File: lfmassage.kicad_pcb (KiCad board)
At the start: 2 copper layers, 63 x 55 mm, 47 parts, among them J1 Batt, J2 OUT, J3 ESP_DEVKITC, Q1 BFS20W, Q2 BC856B,215, Q3 BC856B,215, Q4 BC856B,215, Q5 BC856B,215, Q6 BC846,215, Q7 BC846,215, Q8 BC846,215, SW1 NW3-A03-05, SW2 SW_Push, SW3 SW_Push, SW4 SW_Push, U1 USB_CType_6Pin, U2 MCP73831

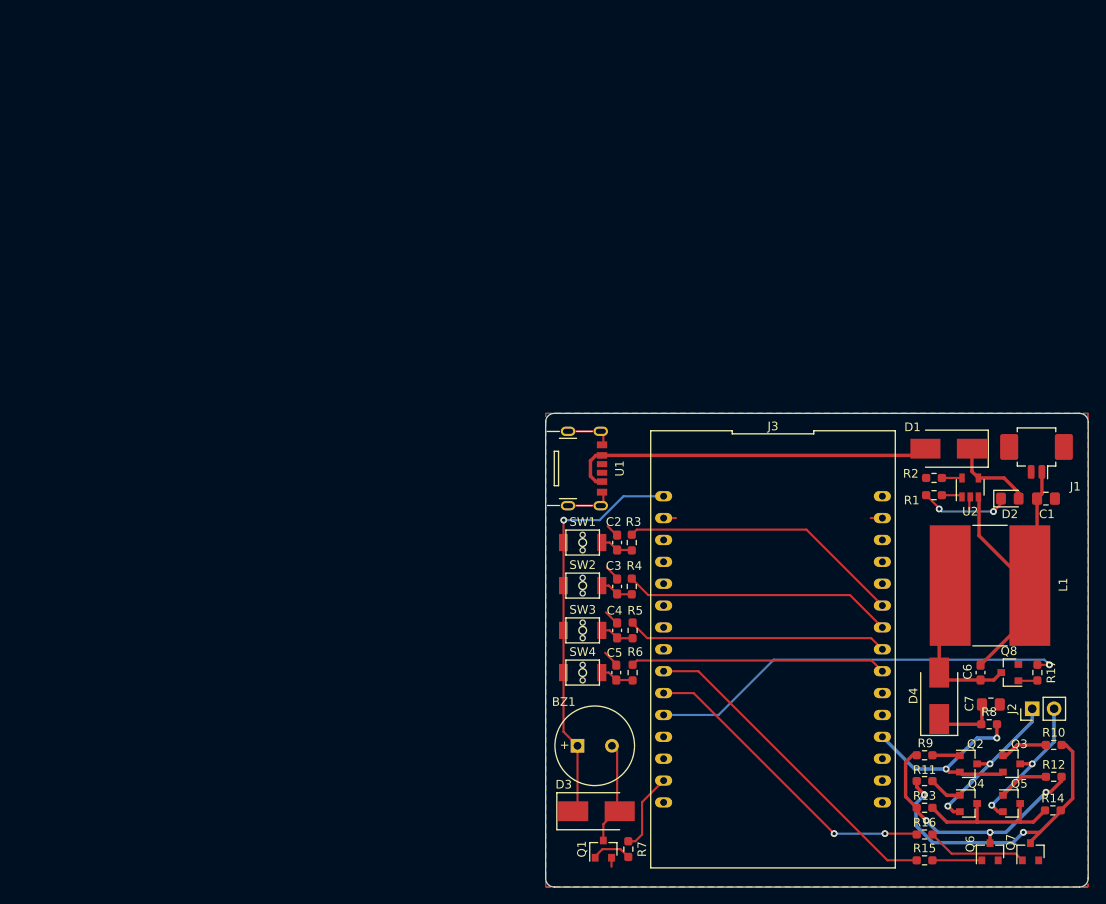
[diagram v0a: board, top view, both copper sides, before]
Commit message: 2021-09-26
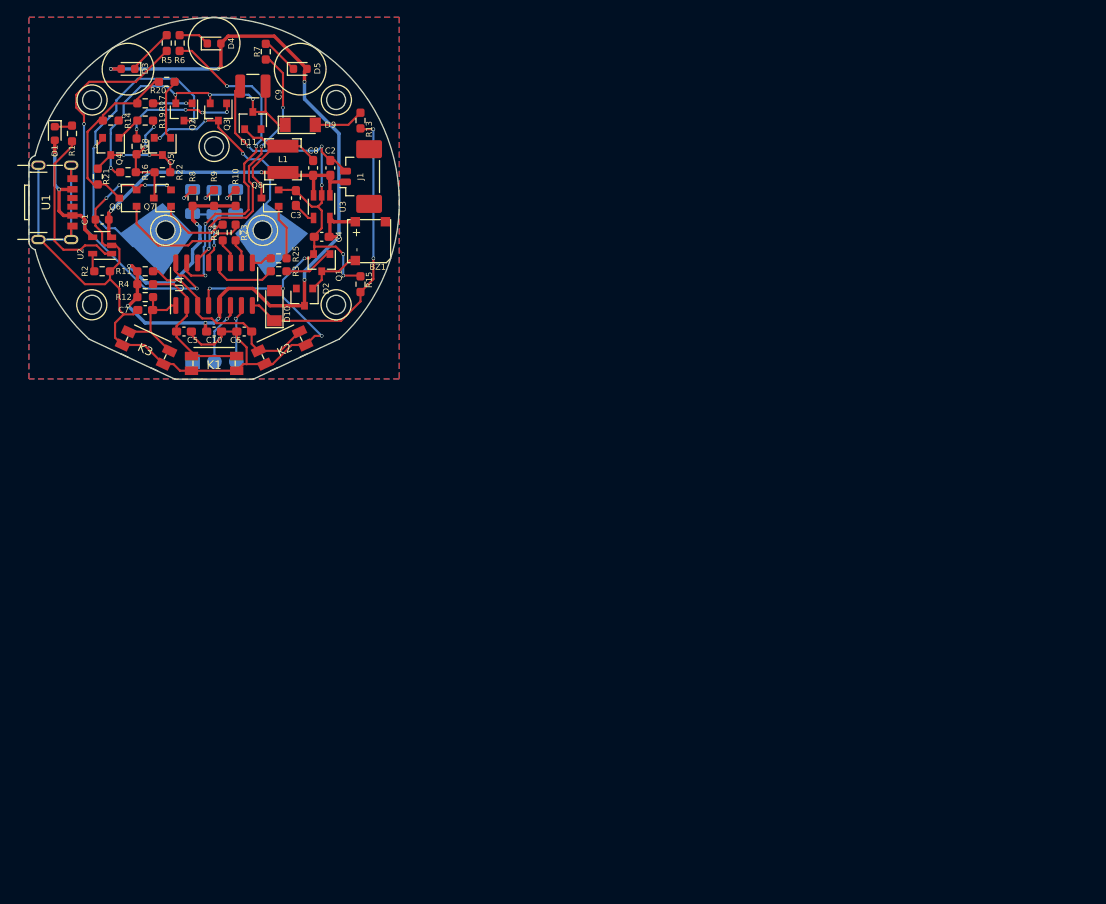
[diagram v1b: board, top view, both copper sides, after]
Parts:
- removed SW1: NW3-A03-05, ali_Switch:NW3-A03-05
- removed SW2, SW3, SW4: SW_Push, ali_Switch:NW3-A03-05
- added C10: 10uF/1608, Capacitor_SMD:C_0603_1608Metric_Pad1.08x0.95mm_HandSolder, F.Cu at (21.5, 36.5)
- added C8: 10nF, Capacitor_SMD:C_0603_1608Metric_Pad1.08x0.95mm_HandSolder, F.Cu at (33.0, 17.5)
- added C9: 10uF/3225, Capacitor_SMD:C_1210_3225Metric, F.Cu at (26.0, 8.00)
- added D10: Zenor/3.3V, Diode_SMD:D_MiniMELF, F.Cu at (28.5, 33.5)
- added D11: BAT54, Diode_SMD:D_SOT-23_ANK, F.Cu at (26.0, 12.0)
- added D5: LED/1608, LED_SMD:LED_0603_1608Metric, F.Cu at (31.5, 6.00)
- added D6: RED, LED_SMD:LED_1206_3216Metric, B.Cu at (19.0, 21.4)
- added D7: IR, LED_SMD:LED_1206_3216Metric, B.Cu at (21.5, 21.5)
- added D8: RED, LED_SMD:LED_1206_3216Metric, B.Cu at (24.0, 21.4)
- added D9: Zenor/47V, Diode_SMD:D_MiniMELF, F.Cu at (31.5, 12.5)
- added K1: MODE, Button_Switch_SMD:Panasonic_EVQPUJ_EVQPUA, F.Cu at (21.5, 40.2)
- added K2: +, Button_Switch_SMD:Panasonic_EVQPUJ_EVQPUA, F.Cu at (29.4, 38.4)
- added K3: -, Button_Switch_SMD:Panasonic_EVQPUJ_EVQPUA, F.Cu at (13.6, 38.4)
- added R18: 33k, Resistor_SMD:R_0603_1608Metric_Pad0.98x0.95mm_HandSolder, F.Cu at (12.5, 15.0)
- added R19: 33k, Resistor_SMD:R_0603_1608Metric_Pad0.98x0.95mm_HandSolder, F.Cu at (13.5, 12.0)
- added R20: 33k, Resistor_SMD:R_0603_1608Metric_Pad0.98x0.95mm_HandSolder, F.Cu at (16.0, 7.50)
- added R21: 33k, Resistor_SMD:R_0603_1608Metric_Pad0.98x0.95mm_HandSolder, F.Cu at (8.00, 18.5)
- added R22: 0, Resistor_SMD:R_0603_1608Metric_Pad0.98x0.95mm_HandSolder, F.Cu at (15.5, 18.0)
- added R23: 100, Resistor_SMD:R_0603_1608Metric_Pad0.98x0.95mm_HandSolder, F.Cu at (24.0, 25.0)
- added R24: 100, Resistor_SMD:R_0603_1608Metric_Pad0.98x0.95mm_HandSolder, F.Cu at (22.5, 25.0)
- added R25: 1k, Resistor_SMD:R_0603_1608Metric_Pad0.98x0.95mm_HandSolder, F.Cu at (29.0, 28.0)
- added REF**: MountingHole_2.2mm_M2, MountingHole:MountingHole_2.2mm_M2, F.Cu at (7.33, 33.4)
- added REF**: MountingHole_2.2mm_M2, MountingHole:MountingHole_2.2mm_M2, F.Cu at (7.33, 9.61)
- added REF**: MountingHole_2.2mm_M2, MountingHole:MountingHole_2.2mm_M2, F.Cu at (35.7, 33.4)
- added REF**: MountingHole_2.2mm_M2, MountingHole:MountingHole_2.2mm_M2, F.Cu at (35.7, 9.61)
- added REF**: MountingHole_2.2mm_M2, MountingHole:MountingHole_2.2mm_M2, F.Cu at (21.5, 15.0)
- added REF**: MountingHole_2.2mm_M2, MountingHole:MountingHole_2.2mm_M2, F.Cu at (27.1, 24.8)
- added REF**: MountingHole_2.2mm_M2, MountingHole:MountingHole_2.2mm_M2, F.Cu at (15.9, 24.8)
- added U3: MIC5318-2.8YD5-TR, Package_TO_SOT_SMD:TSOT-23-5, F.Cu at (34.0, 22.0)
- added U4: EFM8BB10F8G-A-SOIC16, Package_SO:SOIC-16_3.9x9.9mm_P1.27mm, F.Cu at (21.5, 31.0)
- BZ1: value IMT09B2703P -> BST-5533S; footprint Buzzer_Beeper:MagneticBuzzer_PUI_AT-0927-TT-6-R -> buzzer:BST-5533S
- C1: value 10uF/2012 -> 10uF/1608; footprint Capacitor_SMD:C_0805_2012Metric_Pad1.18x1.45mm_HandSolder -> Capacitor_SMD:C_0603_1608Metric
- C3: value 100nF/1608 -> 10nF/1608
- C6: value 10nF -> 100nF/1608
- C7: value 10uF/2012 -> 100nF/1608; footprint Capacitor_SMD:C_0805_2012Metric_Pad1.18x1.45mm_HandSolder -> Capacitor_SMD:C_0603_1608Metric_Pad1.08x0.95mm_HandSolder
- D1, D3, D4: value SK24/SMB -> LED/1608; footprint Diode_SMD:D_SMB_Handsoldering -> LED_SMD:LED_0603_1608Metric
- D2: value LED/2012 -> BAT54; footprint LED_SMD:LED_0805_2012Metric_Pad1.15x1.40mm_HandSolder -> Diode_SMD:D_SOT-23_ANK
- J1: footprint Connector_Molex:Molex_PicoBlade_53261-0271_1x02-1MP_P1.25mm_Horizontal -> Connector_Molex:Molex_PicoBlade_53398-0271_1x02-1MP_P1.25mm_Vertical
- J2: value OUT -> electrode; footprint Connector_PinHeader_2.54mm:PinHeader_1x02_P2.54mm_Vertical -> lfmassage_pad:electrode; moved to B.Cu
- J3: value ESP_DEVKITC -> ISP; footprint espressif:ESP32_DEVKITC -> Connector_PinHeader_2.54mm:PinHeader_1x03_P2.54mm_Vertical; moved to B.Cu
- L1: footprint inductor:SDR1307-102KL -> Inductor_SMD:L_Bourns-SRN4018
- Q1: value BFS20W -> S8050
- R10: value 33k -> 220
- R11, R12: value 33k -> 1k
- R13: value 33k -> 1M
- R15: value 1k -> 100k
- R16, R17: value 1k -> 33k
- R3: value 1k -> 150
- R5, R6: value 1k -> 560
- R7: value 100 -> 560
- R8: value 0 -> 220
- R9: value 33k -> 100
- moved R14 135.6 mm to (9.50, 12.0)
- moved Q7 126.2 mm to (15.5, 21.0), turned to 180 degrees
- moved Q6 125.6 mm to (11.5, 21.0), turned to 180 degrees
- moved Q4 125.5 mm to (9.50, 15.0), turned to 270 degrees
- moved Q5 124.7 mm to (15.5, 15.0), turned to 270 degrees
- moved R17 122.9 mm to (13.5, 10.0), turned to 180 degrees
- moved R16 120.3 mm to (11.5, 18.0), turned to 0 degrees
- moved R12 119.3 mm to (13.5, 32.5), turned to 180 degrees
- moved Q3 119.2 mm to (22.0, 11.0), turned to 270 degrees
- moved Q2 118.4 mm to (18.0, 11.0), turned to 270 degrees
- moved C1 114.3 mm to (8.50, 23.5), turned to 180 degrees
- moved R10 114.3 mm to (24.0, 21.0), turned to 90 degrees
- moved D4 113.3 mm to (21.5, 3.05), turned to 0 degrees
- moved J2 111.7 mm to (21.5, 21.6), turned to 180 degrees
- moved R8 110.9 mm to (19.0, 21.0), turned to 90 degrees
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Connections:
- BZ1 pad 1: +3V3 -> VCC
- C2 pad 1: Net-(C2-Pad1) -> BATT
- C4 pad 1: Net-(C4-Pad1) -> VCC
- C5 pad 1: Net-(C5-Pad1) -> P0.1(MODE)
- C6 pad 1: BATT -> P0.0(+)
- C6 pad 2: Net-(C6-Pad2) -> Earth
- C7 pad 1: /Boost Converter/HIGH_VOLTAGE -> P0.2(-)
- D2 pad 1: Net-(D2-Pad1) -> VCC
- D2 pad 2: Net-(D1-Pad1) -> Net-(BZ1-Pad2)
- D3 pad 1: +3V3 -> Net-(D3-Pad1)
- D3 pad 2: Net-(BZ1-Pad2) -> VCC
- D4 pad 1: /Boost Converter/HIGH_VOLTAGE -> Net-(D4-Pad1)
- D4 pad 2: Net-(C6-Pad2) -> VCC
- J2 pad 1: /H-Bridge/OUTH -> /H-Bridge/OUTL
- J2 pad 2: /H-Bridge/OUTL -> /H-Bridge/OUTH
- J3 pad 1: +3V3 -> Earth
- J3 pad 2: Earth -> C2CK
- J3 pad 3: Net-(J3-Pad3) -> C2D
- L1 pad 2: Net-(C6-Pad2) -> Net-(C8-Pad2)
- Q2 pad 2: D34 -> /Boost Converter/HIGH_VOLTAGE
- Q3 pad 2: D34 -> /Boost Converter/HIGH_VOLTAGE
- Q8 pad 3: Net-(C6-Pad2) -> Net-(C8-Pad2)
- R1 pad 1: Net-(D2-Pad1) -> Net-(D1-Pad1)
- R10 pad 1: Net-(Q3-Pad1) -> VCC
- R10 pad 2: Net-(Q7-Pad3) -> Net-(D8-Pad2)
- R11 pad 1: Net-(Q4-Pad1) -> P0.0(+)
- R11 pad 2: Net-(Q7-Pad3) -> VCC
- R12 pad 1: Net-(Q5-Pad1) -> P0.2(-)
- R12 pad 2: Net-(Q6-Pad3) -> VCC
- R13 pad 1: Net-(Q6-Pad3) -> P1.3(SENS)
- R13 pad 2: Net-(Q4-Pad3) -> Net-(D9-Pad2)
- R14 pad 1: Net-(Q7-Pad3) -> /Boost Converter/HIGH_VOLTAGE
- R14 pad 2: Net-(Q4-Pad3) -> Net-(Q6-Pad3)
- R15 pad 1: Net-(Q6-Pad1) -> Earth
- R15 pad 2: D18 -> P1.3(SENS)
- R16 pad 1: Net-(Q7-Pad1) -> /Boost Converter/HIGH_VOLTAGE
- R16 pad 2: D19 -> Net-(Q7-Pad3)
- R17 pad 1: Net-(Q8-Pad1) -> Net-(Q2-Pad1)
- R17 pad 2: D21 -> Net-(Q6-Pad3)
- R3 pad 1: Net-(C2-Pad1) -> Net-(Q1-Pad1)
- R3 pad 2: D27 -> P0.7(BUZZER)
- R4 pad 1: Net-(C3-Pad1) -> P0.1(MODE)
- R4 pad 2: D26 -> VCC
- R5 pad 1: Net-(C4-Pad1) -> Net-(D3-Pad1)
- R5 pad 2: D25 -> P0.3(RED)
- R6 pad 1: Net-(C5-Pad1) -> Net-(D4-Pad1)
- R6 pad 2: D33 -> P0.4(GRN)
- R7 pad 1: Net-(Q1-Pad1) -> Net-(D5-Pad1)
- R7 pad 2: D22 -> P0.5(BLU)
- R8 pad 1: /Boost Converter/HIGH_VOLTAGE -> VCC
- R8 pad 2: D34 -> Net-(D6-Pad2)
- R9 pad 1: Net-(Q2-Pad1) -> VCC
- R9 pad 2: Net-(Q6-Pad3) -> Net-(D7-Pad2)
- U2 pad 4: Net-(D1-Pad1) -> VBUS
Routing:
- net Earth: track 23.7 -> 177.5 mm, vias 0 -> 13
- net VCC: track 0.00 -> 119.6 mm, vias 0 -> 10
- net D21: track 49.4 -> 0.00 mm, vias 1 -> 0
- net P0.3(RED): track 0.00 -> 48.8 mm, vias 0 -> 2
- net +3V3: track 47.5 -> 0.00 mm, vias 1 -> 0
- net P0.4(GRN): track 0.00 -> 41.1 mm, vias 0 -> 4
- net D18: track 38.5 -> 0.00 mm
- net P1.3(SENS): track 0.00 -> 36.4 mm, vias 0 -> 2
- net D19: track 36.2 -> 0.00 mm, vias 2 -> 0
- net D27: track 33.0 -> 0.00 mm
- net D26: track 31.6 -> 0.00 mm
- net P0.5(BLU): track 0.00 -> 31.0 mm, vias 0 -> 4
- net D25: track 30.4 -> 0.00 mm
- net /Boost Converter/HIGH_VOLTAGE: track 7.47 -> 37.7 mm, vias 0 -> 5
- net D33: track 29.7 -> 0.00 mm
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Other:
- board size 63 x 55 mm -> 43 x 42 mm
- net class Default: via_dia 0.8 -> 0.4; via_drill 0.4 -> 0.3
- net class HV added: clearance 0.6, trace_width 0.25, via_dia 0.4, via_drill 0.3
- net class pwr: clearance 0.6 -> 0.2; via_dia 0.8 -> 0.4; via_drill 0.4 -> 0.3
